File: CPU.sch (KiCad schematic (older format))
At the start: 20 parts, among them J301 Molex+Microfit3-Dual4-90, J302 Conn_02x18_Odd_Even, U301 MC9S12XEP100, Y301 16mHz

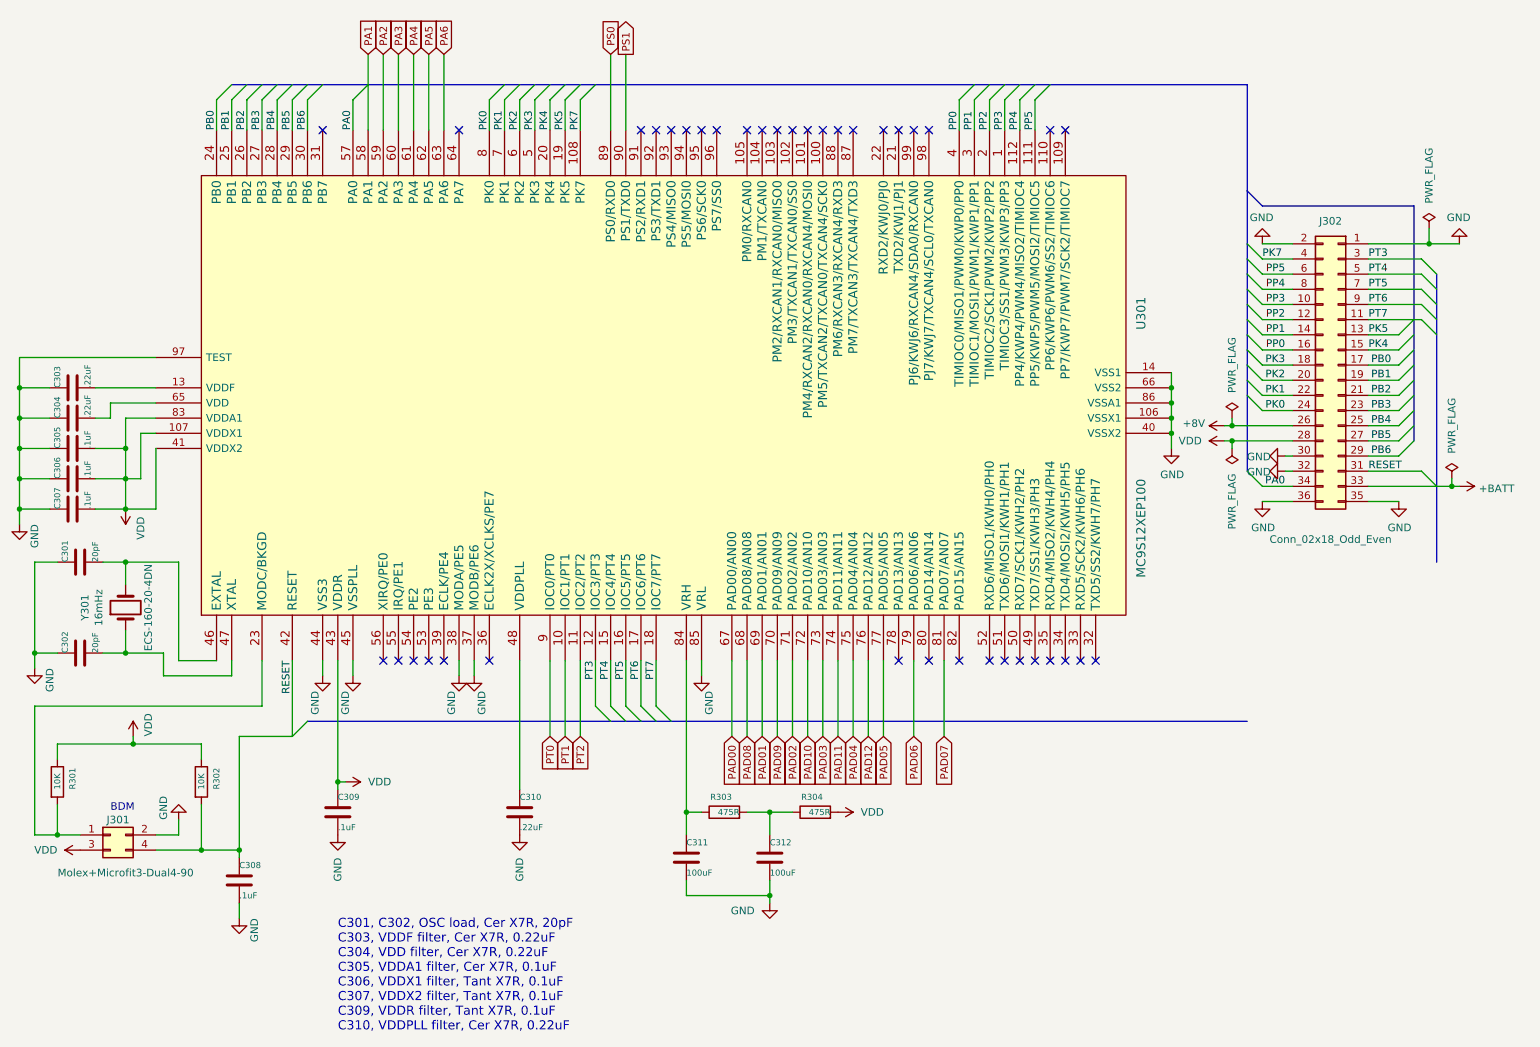
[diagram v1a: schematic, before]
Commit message: Add files via upload
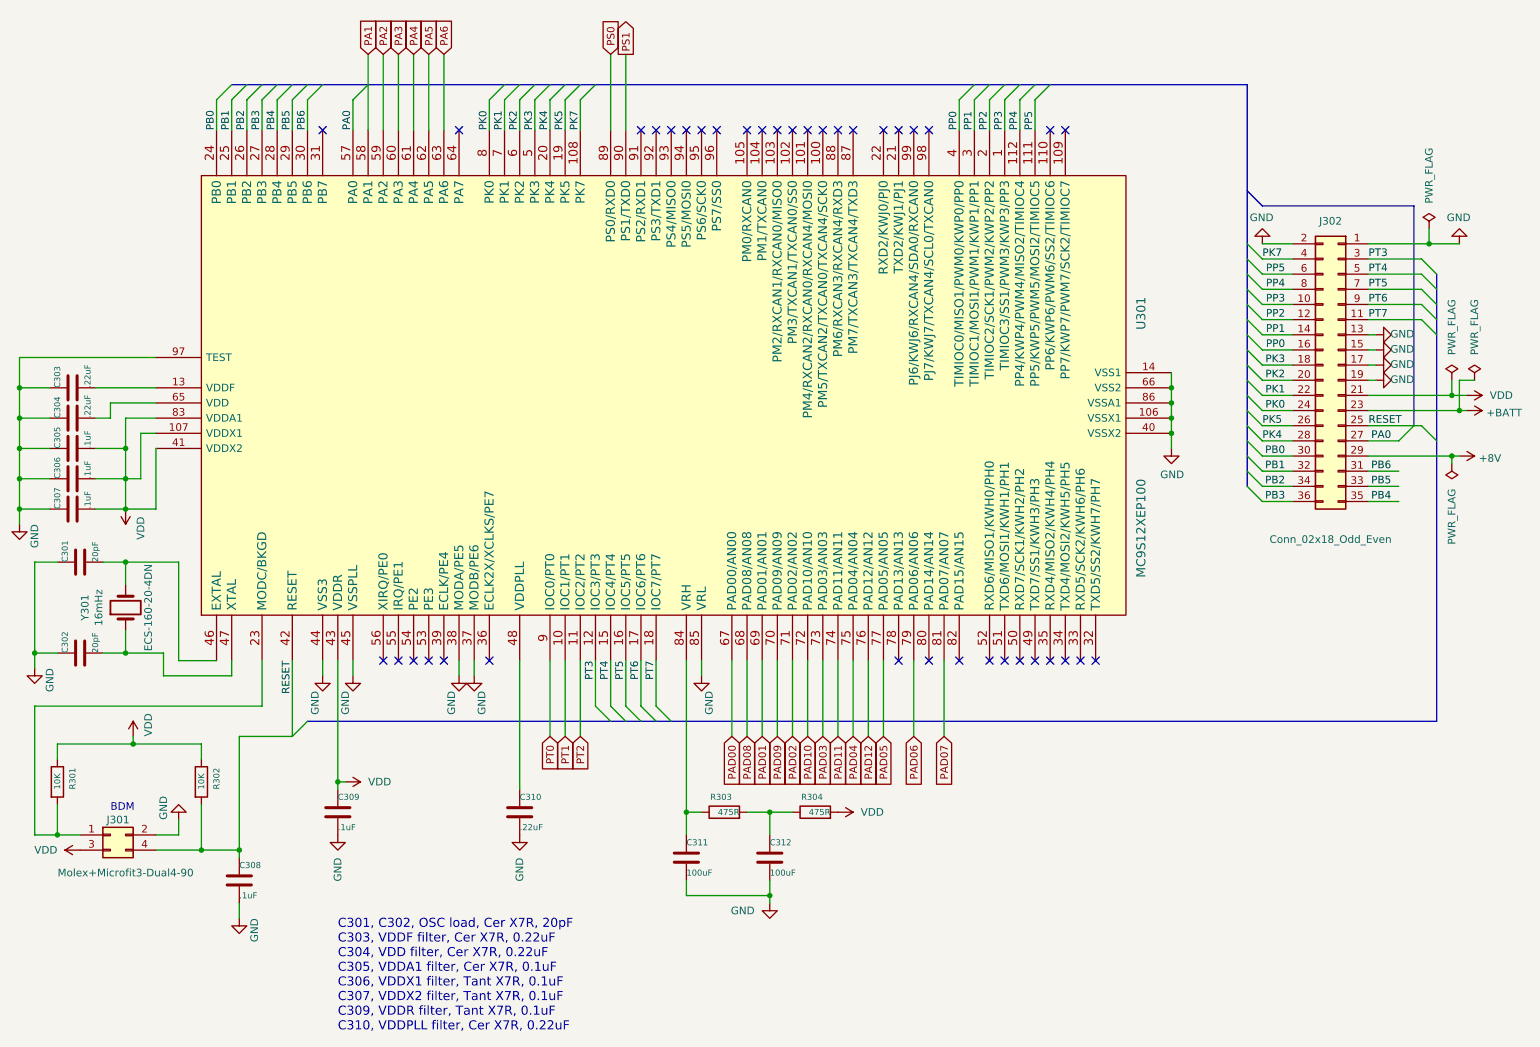
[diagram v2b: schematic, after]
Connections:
- net +8V: now also J302.29 (Pin_29); no longer J302.26 (Pin_26)
- net +BATT: now also J302.23 (Pin_23); no longer J302.33 (Pin_33)
- net GND: now also J302.13 (Pin_13), J302.15 (Pin_15), J302.17 (Pin_17), J302.19 (Pin_19); no longer J302.30 (Pin_30), J302.32 (Pin_32), J302.35 (Pin_35), J302.36 (Pin_36)
- net PA0: now also J302.27 (Pin_27); no longer J302.34 (Pin_34)
- net PB0: now also J302.30 (Pin_30); no longer J302.17 (Pin_17)
- net PB1: now also J302.32 (Pin_32); no longer J302.19 (Pin_19)
- net PB2: now also J302.34 (Pin_34); no longer J302.21 (Pin_21)
- net PB3: now also J302.36 (Pin_36); no longer J302.23 (Pin_23)
- net PB4: now also J302.35 (Pin_35); no longer J302.25 (Pin_25)
- net PB5: now also J302.33 (Pin_33); no longer J302.27 (Pin_27)
- net PB6: now also J302.31 (Pin_31); no longer J302.29 (Pin_29)
- net PK4: now also J302.28 (Pin_28); no longer J302.15 (Pin_15)
- net PK5: now also J302.26 (Pin_26); no longer J302.13 (Pin_13)
- net RESET: now also J302.25 (Pin_25); no longer J302.31 (Pin_31)
- net VDD: now also J302.21 (Pin_21); no longer J302.28 (Pin_28)
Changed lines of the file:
@@
 L power:PWR_FLAG #FLG?
 U 1 1 5EF75985
-P 8600 3750
+P 10200 3500
 AR Path="/5EF75985" Ref="#FLG?"  Part="1"
 AR Path="/5EF2B07F/5EF75985" Ref="#FLG0302"  Part="1"
-F 0 "#FLG0302" H 8600 3825 50  0001 C CNN
-F 1 "PWR_FLAG" V 8600 4100 50  0000 C CNN
-F 2 "" H 8600 3750 50  0001 C CNN
-F 3 "~" H 8600 3750 50  0001 C CNN
-	1    8600 3750
+F 0 "#FLG0302" H 10200 3575 50  0001 C CNN
+F 1 "PWR_FLAG" V 10200 3850 50  0000 C CNN
+F 2 "" H 10200 3500 50  0001 C CNN
+F 3 "~" H 10200 3500 50  0001 C CNN
+	1    10200 3500
 	1    0    0    -1
 $EndComp
@@
 L power:PWR_FLAG #FLG?
 U 1 1 5EF7598B
-P 8600 3950
+P 10050 4050
 AR Path="/5EF7598B" Ref="#FLG?"  Part="1"
 AR Path="/5EF2B07F/5EF7598B" Ref="#FLG0303"  Part="1"
-F 0 "#FLG0303" H 8600 4025 50  0001 C CNN
-F 1 "PWR_FLAG" V 8600 4300 50  0000 C CNN
-F 2 "" H 8600 3950 50  0001 C CNN
-F 3 "~" H 8600 3950 50  0001 C CNN
-	1    8600 3950
+F 0 "#FLG0303" H 10050 4125 50  0001 C CNN
+F 1 "PWR_FLAG" V 10050 4400 50  0000 C CNN
+F 2 "" H 10050 4050 50  0001 C CNN
+F 3 "~" H 10050 4050 50  0001 C CNN
+	1    10050 4050
 	-1   0    0    1
 $EndComp
@@
 Text Label 8950 3300 2    50   ~ 0
 PP0
+Text Label 9650 3900 2    50   ~ 0
+PA0
+Text Label 9650 4300 2    50   ~ 0
+PB4
+Text Label 8950 4100 2    50   ~ 0
+PB1
+Text Label 8950 4000 2    50   ~ 0
+PB0
 Text Label 8950 4200 2    50   ~ 0
-PA0
-Text Label 9650 3800 2    50   ~ 0
-PB4
-Text Label 9650 3500 2    50   ~ 0
-PB1
-Text Label 9650 3400 2    50   ~ 0
-PB0
-Text Label 9650 3600 2    50   ~ 0
 PB2
-Text Label 9650 3700 2    50   ~ 0
+Text Label 8950 4300 2    50   ~ 0
 PB3
 Text Label 9500 3100 0    50   ~ 0
@@
 Text Label 9500 2700 0    50   ~ 0
 PT3
-Wire Wire Line
-	9500 3200 9700 3200
-Wire Wire Line
-	9500 3300 9700 3300
-Wire Wire Line
-	9500 3400 9700 3400
-Wire Wire Line
-	9500 4300 9700 4300
-Entry Wire Line
-	9700 3700 9800 3600
-Entry Wire Line
-	9700 3200 9800 3100
-Entry Wire Line
-	9700 3300 9800 3200
-Entry Wire Line
-	9700 3400 9800 3300
 $Comp
 L power:+8V #PWR?
 U 1 1 5EF75A14
-P 8550 3800
+P 10100 4000
 AR Path="/5EF75A14" Ref="#PWR?"  Part="1"
 AR Path="/5EF2B07F/5EF75A14" Ref="#PWR0323"  Part="1"
-F 0 "#PWR0323" H 8550 3650 50  0001 C CNN
-F 1 "+8V" V 8565 3928 50  0000 L CNN
-F 2 "" H 8550 3800 50  0001 C CNN
-F 3 "" H 8550 3800 50  0001 C CNN
-	1    8550 3800
-	0    -1   -1   0
+F 0 "#PWR0323" H 10100 3850 50  0001 C CNN
+F 1 "+8V" V 10115 4128 50  0000 L CNN
+F 2 "" H 10100 4000 50  0001 C CNN
+F 3 "" H 10100 4000 50  0001 C CNN
+	1    10100 4000
+	0    1    1    0
 $EndComp
 $Comp
 L power:GND #PWR?
 U 1 1 5EF75A1A
-P 8800 4300
+P 9550 3500
 AR Path="/5EF75A1A" Ref="#PWR?"  Part="1"
 AR Path="/5EF2B07F/5EF75A1A" Ref="#PWR0320"  Part="1"
-F 0 "#PWR0320" H 8800 4050 50  0001 C CNN
-F 1 "GND" H 8805 4127 50  0000 C CNN
-F 2 "" H 8800 4300 50  0001 C CNN
-F 3 "" H 8800 4300 50  0001 C CNN
-	1    8800 4300
-	1    0    0    -1
+F 0 "#PWR0320" H 9550 3250 50  0001 C CNN
+F 1 "GND" V 9555 3327 50  0000 C CNN
+F 2 "" H 9550 3500 50  0001 C CNN
+F 3 "" H 9550 3500 50  0001 C CNN
+	1    9550 3500
+	0    -1   -1   0
 $EndComp
 $Comp
@@
 L power:GND #PWR?
 U 1 1 5EF75A2C
-P 9700 4300
+P 9550 3200
 AR Path="/5EF75A2C" Ref="#PWR?"  Part="1"
 AR Path="/5EF2B07F/5EF75A2C" Ref="#PWR0321"  Part="1"
-F 0 "#PWR0321" H 9700 4050 50  0001 C CNN
-F 1 "GND" H 9705 4127 50  0000 C CNN
-F 2 "" H 9700 4300 50  0001 C CNN
-F 3 "" H 9700 4300 50  0001 C CNN
-	1    9700 4300
-	1    0    0    -1
+F 0 "#PWR0321" H 9550 2950 50  0001 C CNN
+F 1 "GND" V 9555 3027 50  0000 C CNN
+F 2 "" H 9550 3200 50  0001 C CNN
+F 3 "" H 9550 3200 50  0001 C CNN
+	1    9550 3200
+	0    -1   -1   0
 $EndComp
 NoConn ~ 3700 5350
@@
 L power:VDD #PWR?
 U 1 1 5EF75A47
-P 8550 3900
+P 10150 3600
 AR Path="/5EF75A47" Ref="#PWR?"  Part="1"
 AR Path="/5EF2B07F/5EF75A47" Ref="#PWR0324"  Part="1"
-F 0 "#PWR0324" H 8550 3750 50  0001 C CNN
-F 1 "VDD" V 8550 4050 50  0000 L CNN
-F 2 "" H 8550 3900 50  0001 C CNN
-F 3 "" H 8550 3900 50  0001 C CNN
-	1    8550 3900
-	0    -1   -1   0
+F 0 "#PWR0324" H 10150 3450 50  0001 C CNN
+F 1 "VDD" V 10150 3750 50  0000 L CNN
+F 2 "" H 10150 3600 50  0001 C CNN
+F 3 "" H 10150 3600 50  0001 C CNN
+	1    10150 3600
+	0    1    1    0
 $EndComp
 Wire Wire Line
@@
 Text Label 8950 3400 2    50   ~ 0
 PK3
-Text Label 9500 3200 0    50   ~ 0
+Text Label 8800 3800 0    50   ~ 0
 PK5
-Text Label 9500 3300 0    50   ~ 0
+Text Label 8800 3900 0    50   ~ 0
 PK4
 Text Label 8800 2700 0    50   ~ 0
@@
 L power:PWR_FLAG #FLG?
 U 1 1 5F01B122
-P 10050 4150
+P 10050 3500
 AR Path="/5F01B122" Ref="#FLG?"  Part="1"
 AR Path="/5EF2B07F/5F01B122" Ref="#FLG0304"  Part="1"
-F 0 "#FLG0304" H 10050 4225 50  0001 C CNN
-F 1 "PWR_FLAG" V 10050 4500 50  0000 C CNN
-F 2 "" H 10050 4150 50  0001 C CNN
-F 3 "~" H 10050 4150 50  0001 C CNN
-	1    10050 4150
+F 0 "#FLG0304" H 10050 3575 50  0001 C CNN
+F 1 "PWR_FLAG" V 10050 3850 50  0000 C CNN
+F 2 "" H 10050 3500 50  0001 C CNN
+F 3 "~" H 10050 3500 50  0001 C CNN
+	1    10050 3500
 	1    0    0    -1
 $EndComp
@@
 Text GLabel 6700 5850 3    50   Input ~ 0
 PAD07
-Wire Wire Line
-	9500 3500 9700 3500
-Entry Wire Line
-	9700 3500 9800 3400
 Text Label 8950 3100 2    50   ~ 0
 PP2
@@
 L power:+BATT #PWR0322
 U 1 1 5F2B675E
-P 10100 4200
-F 0 "#PWR0322" H 10100 4050 50  0001 C CNN
-F 1 "+BATT" V 10115 4328 50  0000 L CNN
-F 2 "" H 10100 4200 50  0001 C CNN
-F 3 "" H 10100 4200 50  0001 C CNN
-	1    10100 4200
+P 10150 3700
+F 0 "#PWR0322" H 10150 3550 50  0001 C CNN
+F 1 "+BATT" V 10165 3828 50  0000 L CNN
+F 2 "" H 10150 3700 50  0001 C CNN
+F 3 "" H 10150 3700 50  0001 C CNN
+	1    10150 3700
 	0    1    1    0
 $EndComp
@@
 Entry Wire Line
 	2500 1650 2600 1550
-Wire Wire Line
-	9500 3600 9700 3600
 Entry Wire Line
 	8700 3500 8800 3600
-Entry Wire Line
-	9700 3600 9800 3500
-Text Label 9650 3900 2    50   ~ 0
+Text Label 9650 4200 2    50   ~ 0
 PB5
-Text Label 9650 4000 2    50   ~ 0
+Text Label 9650 4100 2    50   ~ 0
 PB6
-Text Label 9500 4100 0    50   ~ 0
+Text Label 9500 3800 0    50   ~ 0
 RESET
 Wire Wire Line
@@
 Connection ~ 600  4350
 Wire Wire Line
-	9500 3700 9700 3700
-Wire Wire Line
-	9500 3800 9700 3800
-Wire Wire Line
 	8800 4300 9000 4300
 Wire Wire Line
@@
 Wire Wire Line
 	9000 3000 8800 3000
-Wire Wire Line
-	9500 3900 9700 3900
-Wire Wire Line
-	9500 4000 9700 4000
 Entry Wire Line
 	8700 2900 8800 3000
@@
 Entry Wire Line
 	9850 3100 9950 3200
-Entry Wire Line
-	9700 3800 9800 3700
-Entry Wire Line
-	9700 3900 9800 3800
-Entry Wire Line
-	9700 4000 9800 3900
-Entry Wire Line
-	9850 4100 9950 4200
 Wire Wire Line
 	9000 4200 8800 4200
-Entry Wire Line
-	8700 4100 8800 4200
-Wire Wire Line
-	9500 4100 9850 4100
-Wire Wire Line
-	10050 4150 10050 4200
-Connection ~ 10050 4200
-Wire Wire Line
-	10050 4200 10100 4200
-Wire Wire Line
-	8550 3800 8600 3800
-Wire Wire Line
-	8550 3900 8600 3900
-Wire Wire Line
-	8600 3950 8600 3900
-Connection ~ 8600 3900
-Wire Wire Line
-	8600 3900 9000 3900
-Wire Wire Line
-	8600 3750 8600 3800
-Connection ~ 8600 3800
-Wire Wire Line
-	8600 3800 9000 3800
 $Comp
 L power:GND #PWR?
 U 1 1 5F233585
-P 8950 4100
+P 9550 3400
 AR Path="/5F233585" Ref="#PWR?"  Part="1"
 AR Path="/5EF2B07F/5F233585" Ref="#PWR0101"  Part="1"
-F 0 "#PWR0101" H 8950 3850 50  0001 C CNN
-F 1 "GND" V 8955 3927 50  0000 C CNN
-F 2 "" H 8950 4100 50  0001 C CNN
-F 3 "" H 8950 4100 50  0001 C CNN
-	1    8950 4100
-	0    1    1    0
+F 0 "#PWR0101" H 9550 3150 50  0001 C CNN
+F 1 "GND" V 9555 3227 50  0000 C CNN
+F 2 "" H 9550 3400 50  0001 C CNN
+F 3 "" H 9550 3400 50  0001 C CNN
+	1    9550 3400
+	0    -1   -1   0
 $EndComp
 $Comp
 L power:GND #PWR?
 U 1 1 5F2556DC
-P 8950 4000
+P 9550 3300
 AR Path="/5F2556DC" Ref="#PWR?"  Part="1"
 AR Path="/5EF2B07F/5F2556DC" Ref="#PWR0102"  Part="1"
-F 0 "#PWR0102" H 8950 3750 50  0001 C CNN
-F 1 "GND" V 8955 3827 50  0000 C CNN
-F 2 "" H 8950 4000 50  0001 C CNN
-F 3 "" H 8950 4000 50  0001 C CNN
-	1    8950 4000
-	0    1    1    0
-$EndComp
-Wire Wire Line
-	9000 4000 8950 4000
-Wire Wire Line
-	9000 4100 8950 4100
+F 0 "#PWR0102" H 9550 3050 50  0001 C CNN
+F 1 "GND" V 9555 3127 50  0000 C CNN
+F 2 "" H 9550 3300 50  0001 C CNN
+F 3 "" H 9550 3300 50  0001 C CNN
+	1    9550 3300
+	0    -1   -1   0
+$EndComp
+Wire Wire Line
+	9000 3800 8800 3800
+Wire Wire Line
+	9000 3900 8800 3900
+Wire Wire Line
+	9000 4000 8800 4000
+Wire Wire Line
+	9000 4100 8800 4100
+Wire Wire Line
+	9500 4100 9700 4100
+Wire Wire Line
+	9500 4200 9700 4200
+Wire Wire Line
+	9500 4300 9700 4300
+Wire Wire Line
+	9500 3100 9850 3100
+Wire Wire Line
+	9550 3200 9500 3200
+Wire Wire Line
+	9550 3300 9500 3300
+Wire Wire Line
+	9550 3400 9500 3400
+Wire Wire Line
+	9550 3500 9500 3500
+Wire Wire Line
+	9500 3900 9700 3900
+Entry Wire Line
+	9850 3800 9950 3900
+Wire Wire Line
+	9500 3600 10050 3600
+Wire Wire Line
+	9500 3700 10100 3700
+Wire Wire Line
+	10050 3500 10050 3600
+Connection ~ 10050 3600
+Wire Wire Line
+	10050 3600 10150 3600
+Wire Wire Line
+	10200 3500 10100 3500
+Wire Wire Line
+	10100 3500 10100 3700
+Connection ~ 10100 3700
+Wire Wire Line
+	10100 3700 10150 3700
+Wire Wire Line
+	9500 4000 10050 4000
+Wire Wire Line
+	10050 4050 10050 4000
+Connection ~ 10050 4000
+Wire Wire Line
+	10050 4000 10100 4000
+Entry Wire Line
+	9700 3900 9800 3800
+Wire Bus Line
+	9800 2350 9800 3800
+Entry Wire Line
+	8800 3800 8700 3700
+Entry Wire Line
+	8800 4000 8700 3900
+Entry Wire Line
+	8700 3800 8800 3900
+Entry Wire Line
+	8700 4000 8800 4100
+Entry Wire Line
+	8700 4100 8800 4200
+Entry Wire Line
+	8700 4200 8800 4300
+Wire Wire Line
+	9500 3800 9850 3800
 Wire Wire Line
 	2900 1350 2900 1850
-Wire Wire Line
-	9500 3100 9850 3100
-Wire Wire Line
-	9500 4200 10050 4200
 Wire Bus Line
-	2500 5750 8700 5750
+	2500 5750 9950 5750
 Wire Bus Line
-	9950 2800 9950 4700
+	9950 2800 9950 5750
 Wire Bus Line
-	9800 2350 9800 3900
-Wire Bus Line
-	8700 1550 8700 4100
+	8700 1550 8700 4200
 Wire Bus Line
 	2000 1550 8700 1550
